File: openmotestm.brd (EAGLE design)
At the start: 24.4 x 34 mm, 49 parts

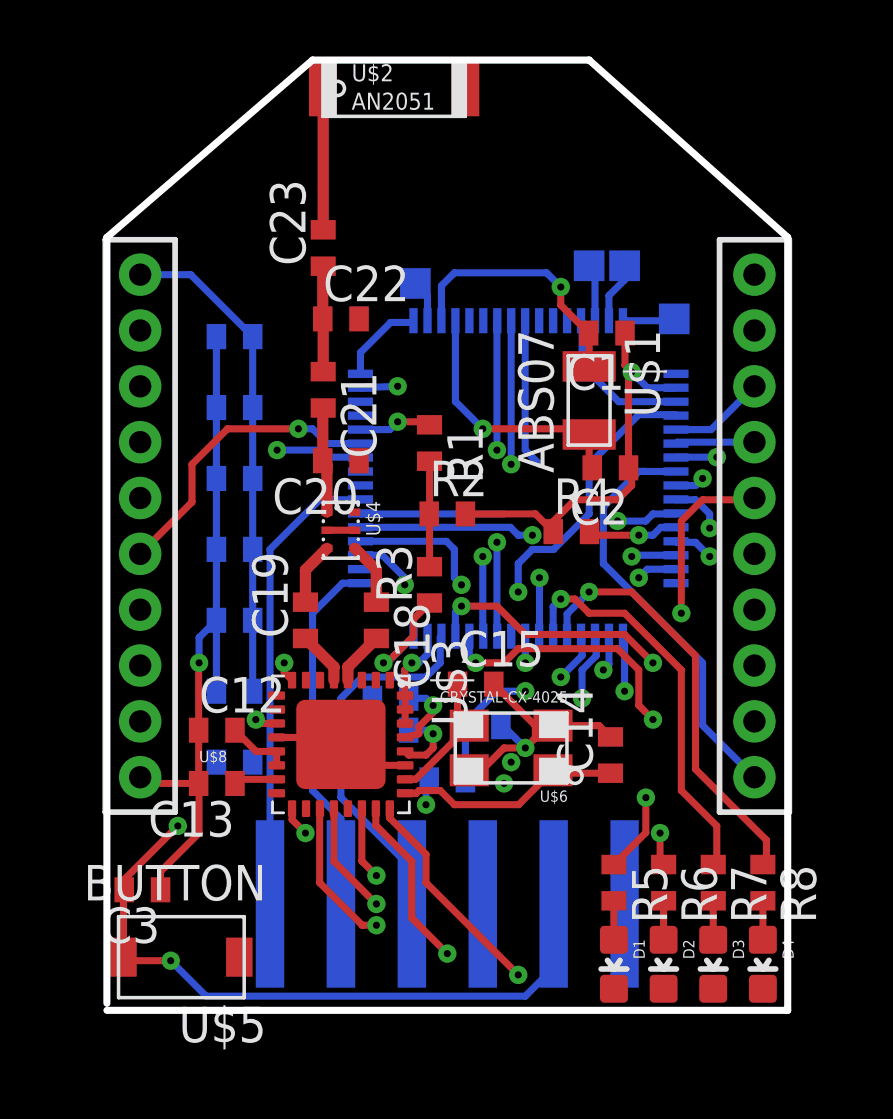
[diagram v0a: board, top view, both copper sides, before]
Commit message: finish the board
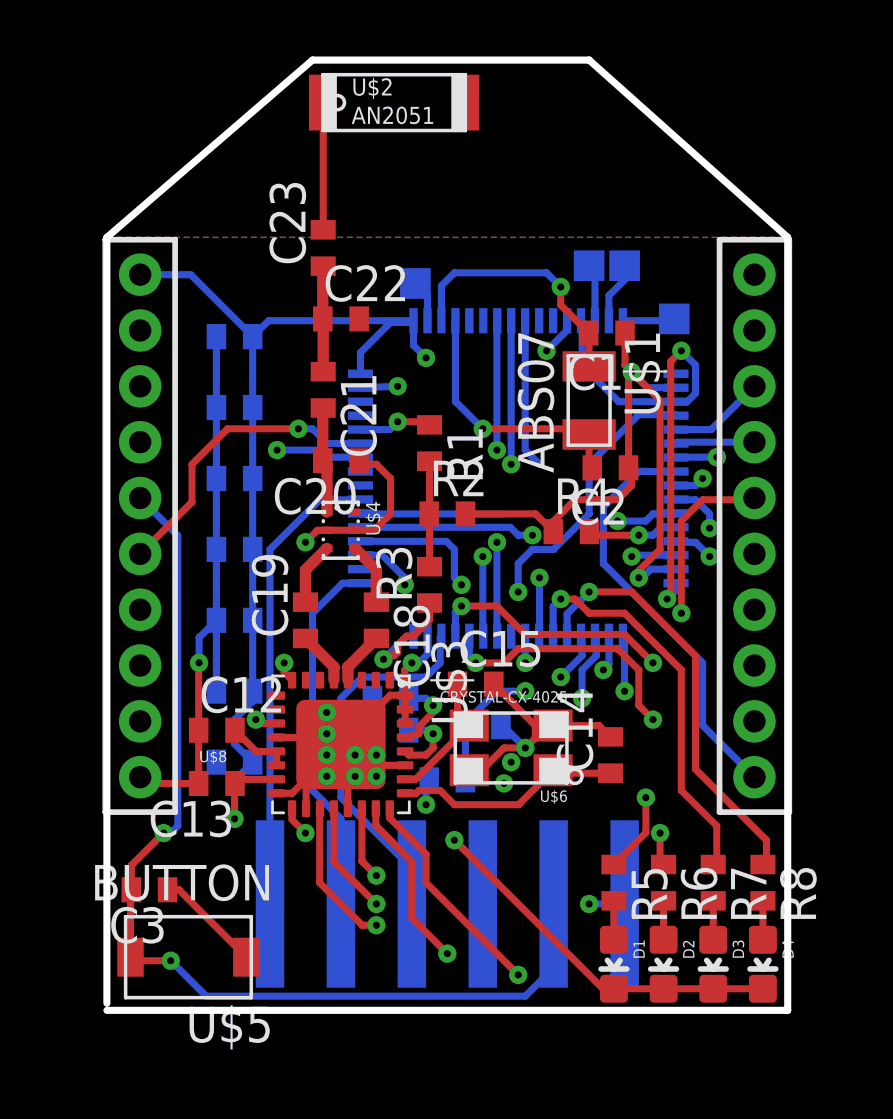
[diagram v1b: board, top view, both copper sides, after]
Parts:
- moved U$2 0.51 mm to (10.8, 78.2)
- moved C3 0.25 mm to (2.03, 50.0)
- moved U$5 0.25 mm to (3.43, 47.6)
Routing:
- net GND: track 62.3 -> 108.2 mm, vias 6 -> 10
- net VCC: track 34.8 -> 66.1 mm, vias 2 -> 7
- added copper zone on layer 1, net GND
- added copper zone on layer 16, net GND
- added copper zone on layer 2, net GND
- added copper zone on layer 15, net VCC
